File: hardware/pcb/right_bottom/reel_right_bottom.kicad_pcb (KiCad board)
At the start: 2 copper layers, 145 x 88.1 mm, 4 parts

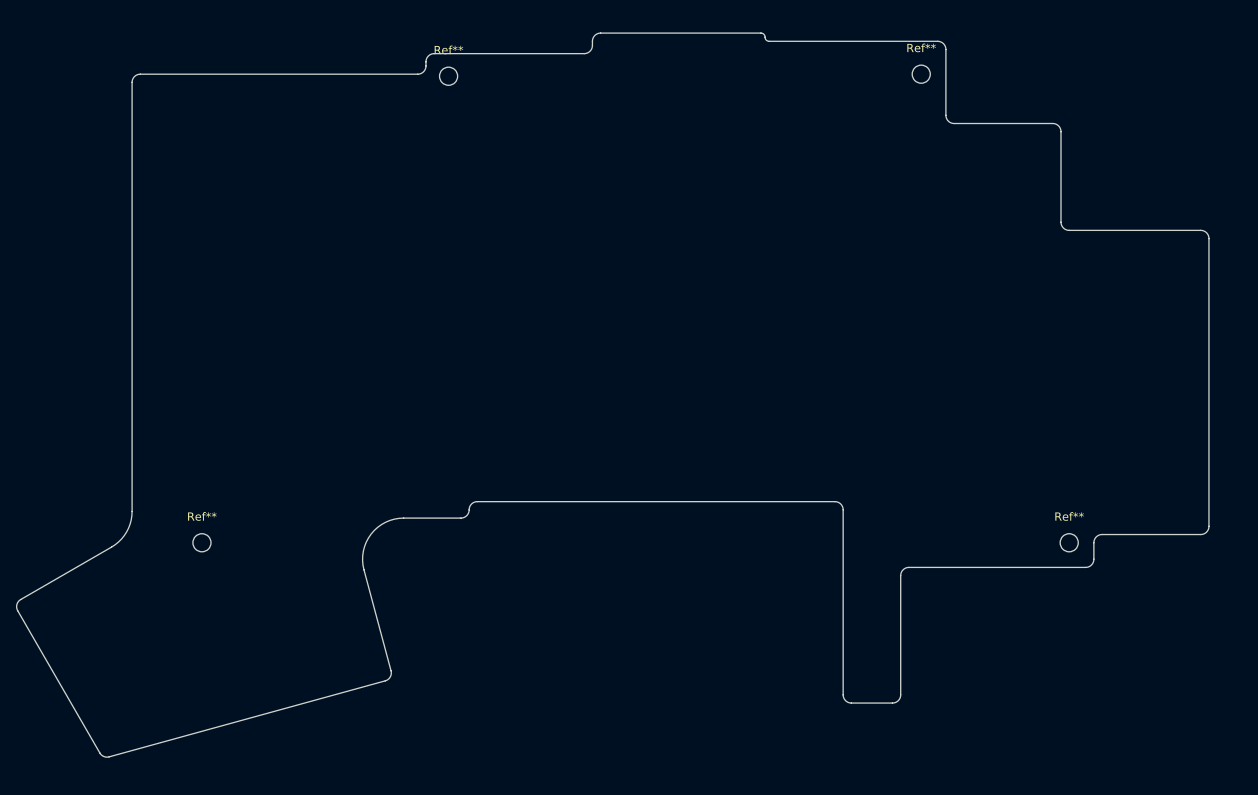
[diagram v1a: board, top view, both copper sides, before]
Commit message: Publish current hardware and fabrication assets
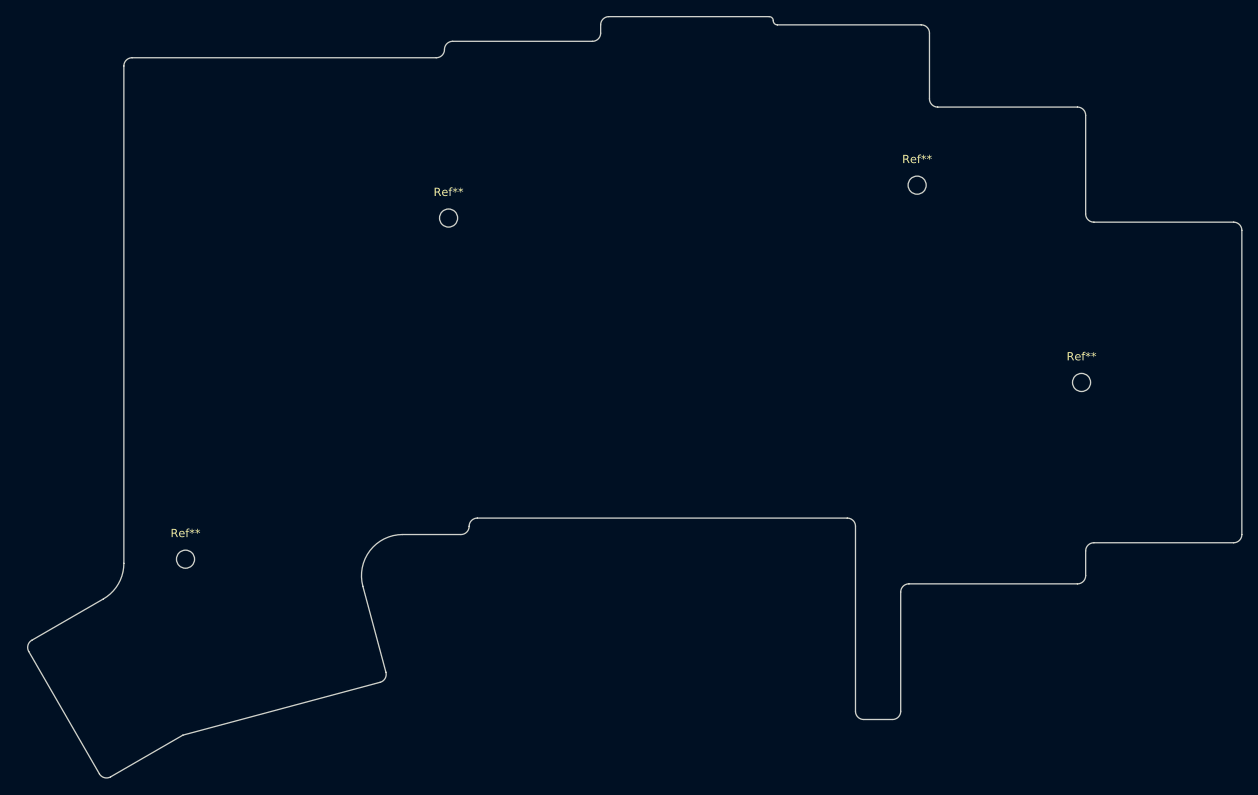
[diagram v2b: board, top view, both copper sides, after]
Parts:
- removed the Ref** at (58.0, 107.5)
- removed the Ref** at (145.5, 50.5)
- removed the Ref** at (88.0, 50.8)
- removed the Ref** at (163.5, 107.5)
- added Ref**: MountingHole_2.2mm_M2, MountingHole:MountingHole_2.2mm_M2, F.Cu at (165.0, 88.0)
- added Ref**: MountingHole_2.2mm_M2, MountingHole:MountingHole_2.2mm_M2, F.Cu at (88.0, 68.0)
- added Ref**: MountingHole_2.2mm_M2, MountingHole:MountingHole_2.2mm_M2, F.Cu at (56.0, 109.5)
- added Ref**: MountingHole_2.2mm_M2, MountingHole:MountingHole_2.2mm_M2, F.Cu at (145.0, 64.0)
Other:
- board size 145 x 88.1 mm -> 147.7 x 92.6 mm
